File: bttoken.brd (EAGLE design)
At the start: 84.5 x 33.5 mm, 53 parts, among them IC1 0, Q1 32k, T1 MMBT3904, X1 FCI-MICRO-USB

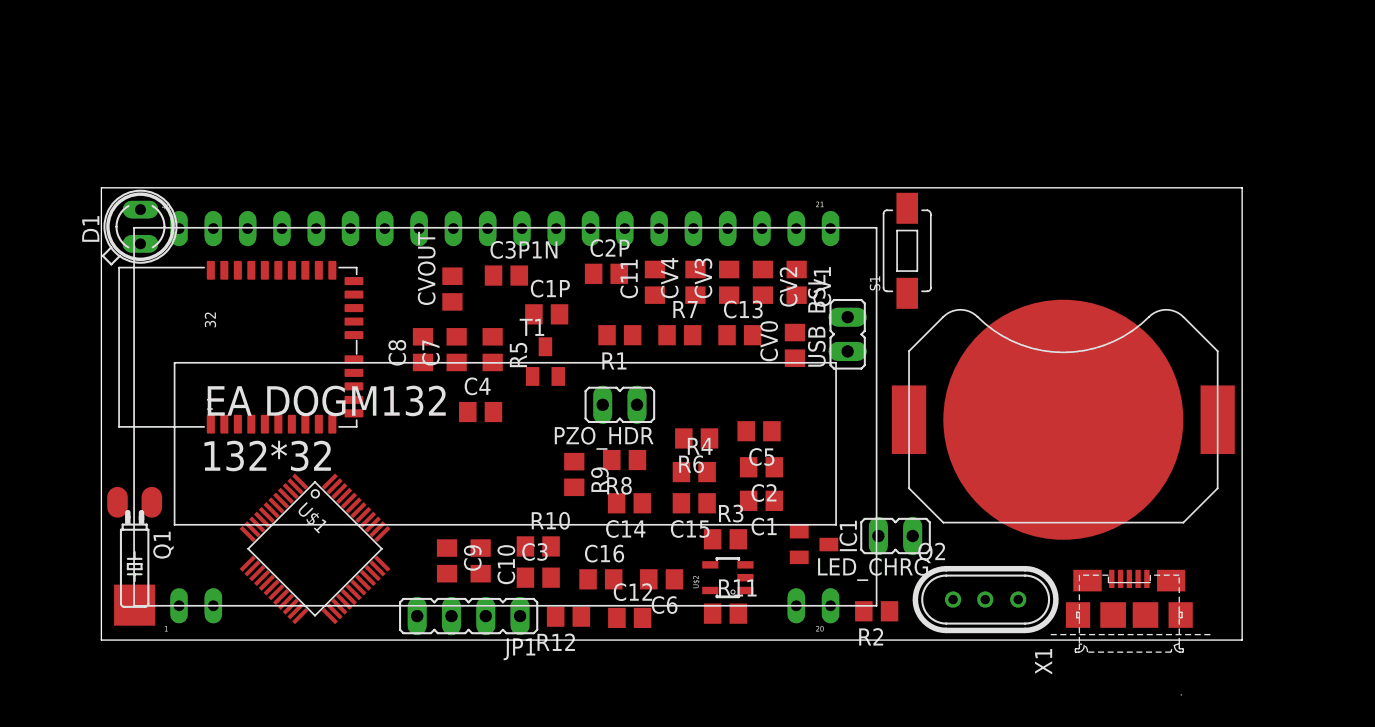
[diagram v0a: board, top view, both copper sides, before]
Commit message: Checkpoint
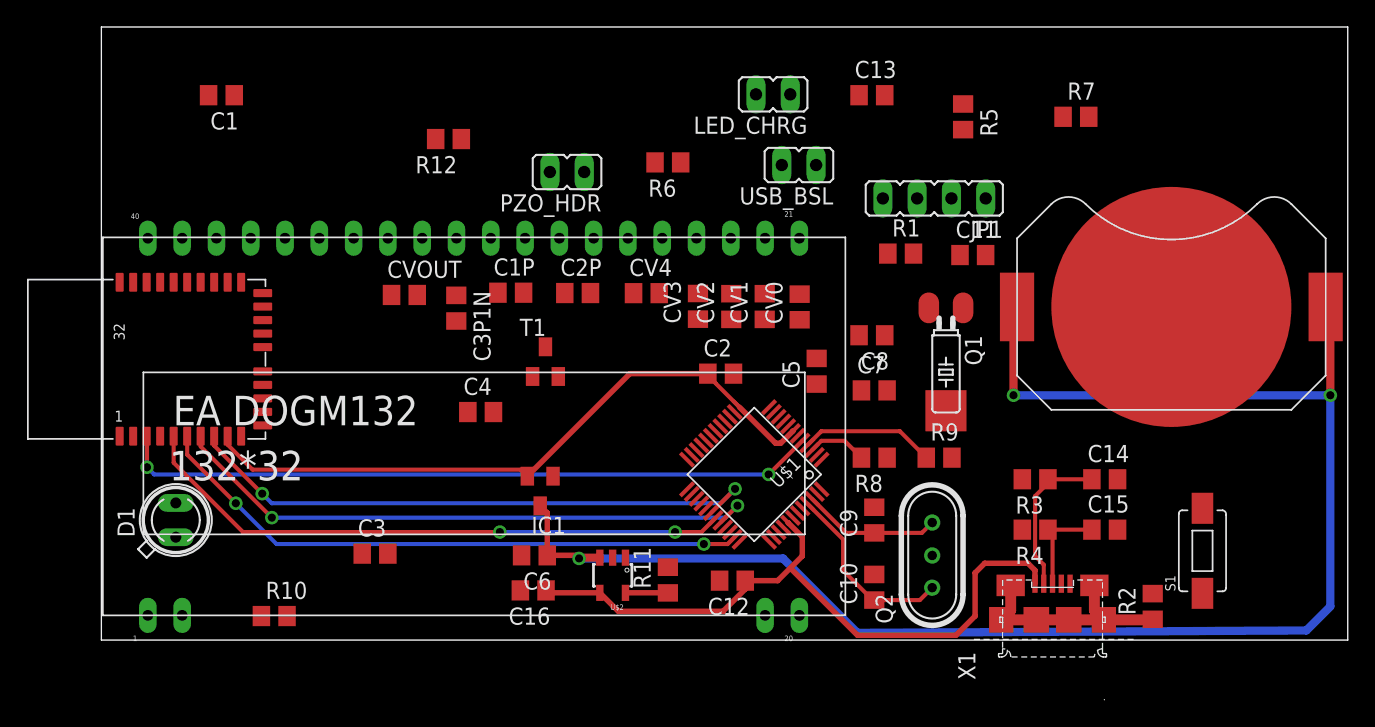
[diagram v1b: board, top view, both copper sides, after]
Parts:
- moved Q1 61.8 mm to (62.6, 24.6)
- moved C1 50.0 mm to (8.89, 40.4)
- moved JP1 46.3 mm to (61.7, 32.7)
- moved R5 38.9 mm to (63.8, 38.8)
- moved R12 36.5 mm to (25.7, 37.1)
- moved C14 35.2 mm to (74.3, 11.9), turned to 0 degrees
- moved LED_CHRG 33.9 mm to (49.8, 40.4)
- moved R7 33.5 mm to (72.2, 38.8)
- moved C8 33.3 mm to (57.1, 22.6), turned to 180 degrees
- moved U$1 33.0 mm to (48.4, 12.3), turned to 225 degrees
- moved C9 31.8 mm to (57.3, 8.89), turned to 90 degrees
- moved S1 31.2 mm to (81.6, 6.61)
- moved C7 31.1 mm to (57.3, 18.5), turned to 0 degrees
- moved C15 30.5 mm to (74.3, 8.18), turned to 0 degrees
- moved C10 29.2 mm to (57.3, 3.91), turned to 90 degrees
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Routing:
- net VBAT: track 0.00 -> 119.1 mm, vias 0 -> 3
- net BTH_RST: track 0.00 -> 52.1 mm, vias 0 -> 2
- net VBUS: track 0.00 -> 50.1 mm
- net VCC: track 0.00 -> 49.2 mm
- net BTH_SEL: track 0.00 -> 44.9 mm, vias 0 -> 2
- net SPI_CLK: track 0.00 -> 44.9 mm, vias 0 -> 2
- net SPI_MISO: track 0.00 -> 44.7 mm, vias 0 -> 2
- net SPI_MOSI: track 0.00 -> 44.0 mm, vias 0 -> 2
- net N$1: track 0.00 -> 16.9 mm
- net XT2IN: track 0.00 -> 13.9 mm
- net N$9: track 0.00 -> 11.7 mm
- net XT2OUT: track 0.00 -> 10.3 mm
- net IR_CTL: track 0.00 -> 10.1 mm
- net N$13: track 0.00 -> 7.40 mm
- net PZO1: track 0.00 -> 4.46 mm
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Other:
- board size 84.5 x 33.5 mm -> 92.3 x 45.4 mm
